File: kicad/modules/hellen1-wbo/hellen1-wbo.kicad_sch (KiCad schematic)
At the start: 65 parts, among them J600 Conn_02x03_Odd_Even, M600 Module-wbo-0.4, Q600 BTS3028, Q601 VNP28N04-E, U600 MCP6004, U601 AD8628, U602 STM32F042K6Tx, U603 REF3033, U604 XC6206P332MR, U605 TJA1051T/3/1J

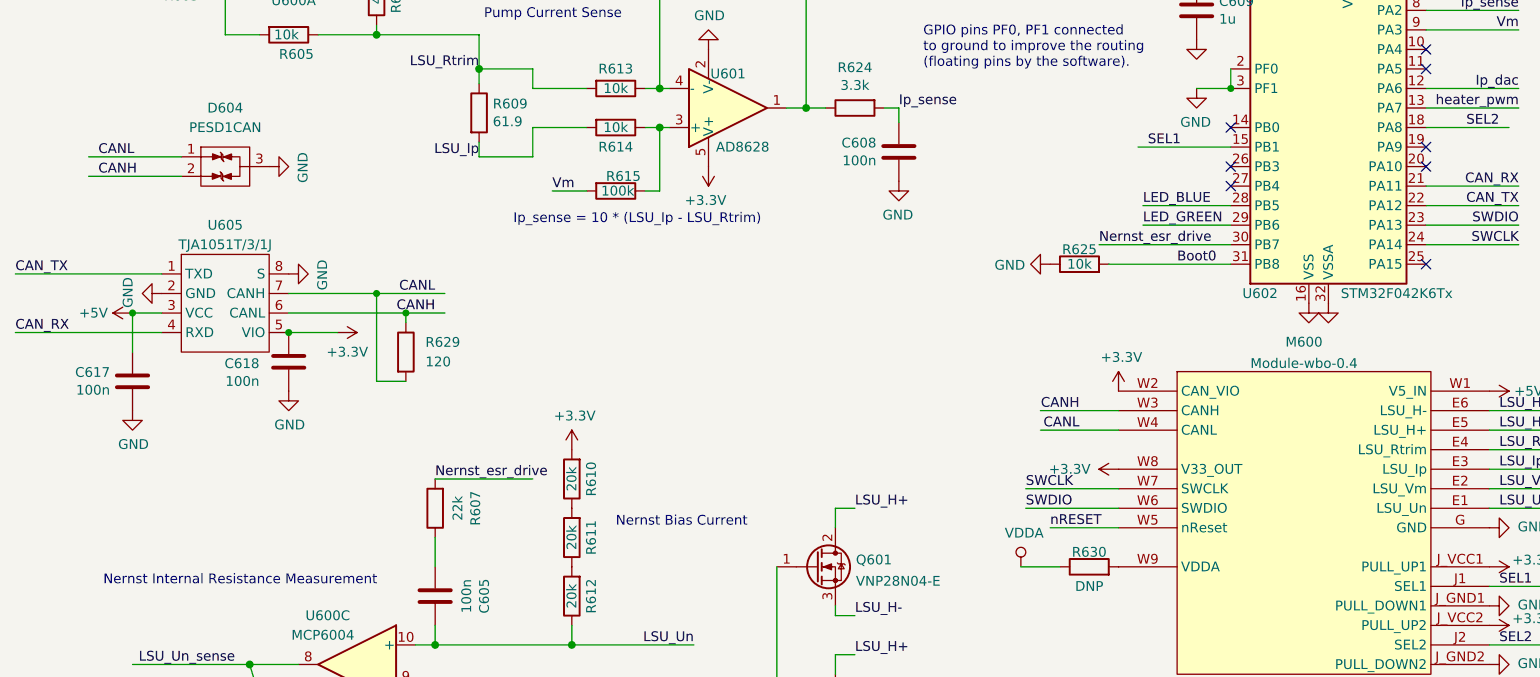
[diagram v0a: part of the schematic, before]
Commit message: rev.0.5
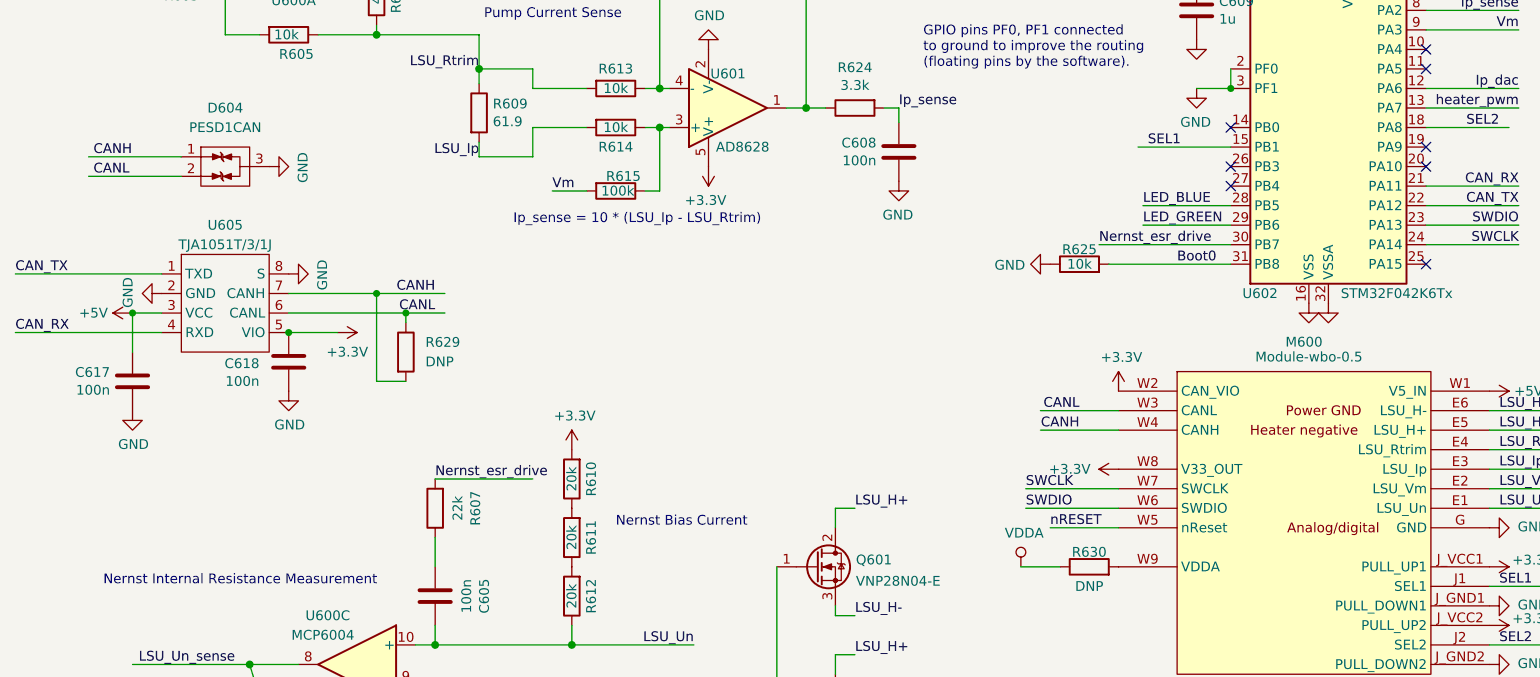
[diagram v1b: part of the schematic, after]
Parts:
- M600: value Module-wbo-0.4 -> Module-wbo-0.5; symbol hellen-one-wbo-0.4:Module-wbo-0.4 -> hellen-one-wbo-0.5:Module-wbo-0.5
- R629: value 120 -> DNP; LCSC C25079 -> (none)
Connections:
- net CANH: now also D604.1 (G), M600.W4 (CANH), R629.2, U605.7 (CANH); no longer D604.2 (D), M600.W3 (CANH), R629.1, U605.6 (CANL)
- net CANL: now also D604.2 (D), M600.W3 (CANL), R629.1, U605.6 (CANL); no longer D604.1 (G), M600.W4 (CANL), R629.2, U605.7 (CANH)
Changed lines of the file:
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@@
     (title "WBO")
     (date "2021-09-28")
-    (rev "0.3")
+    (rev "0.5")
     (company "rusefi.com")
   )
@@
     (effects (font (size 1.27 1.27)) (justify left bottom))
   )
-  (label "CANH" (at 72.39 114.3 180)
+  (label "CANH" (at 72.39 111.76 180)
     (effects (font (size 1.27 1.27)) (justify right bottom))
   )
@@
     (effects (font (size 1.27 1.27)) (justify right bottom))
   )
-  (label "CANH" (at 28.575 96.52 0)
+  (label "CANH" (at 27.94 93.98 0)
     (effects (font (size 1.27 1.27)) (justify left bottom))
   )
@@
     (effects (font (size 1.27 1.27)) (justify left bottom))
   )
-  (label "CANL" (at 28.575 93.98 0)
+  (label "CANL" (at 27.94 96.52 0)
     (effects (font (size 1.27 1.27)) (justify left bottom))
   )
@@
     (effects (font (size 1.27 1.27)) (justify right bottom))
   )
-  (label "CANH" (at 156.21 127 180)
+  (label "CANH" (at 156.21 129.54 180)
     (effects (font (size 1.27 1.27)) (justify right bottom))
   )
-  (label "CANL" (at 72.39 111.76 180)
+  (label "CANL" (at 72.39 114.3 180)
     (effects (font (size 1.27 1.27)) (justify right bottom))
   )
@@
     (effects (font (size 1.27 1.27)) (justify left bottom))
   )
-  (label "CANL" (at 156.21 129.54 180)
+  (label "CANL" (at 156.21 127 180)
     (effects (font (size 1.27 1.27)) (justify right bottom))
   )
@@
     (pin "1")
   )
-  (symbol (lib_id "hellen-one-wbo-0.4:Module-wbo-0.4") (at 168.91 121.92 0) (unit 1)
-    (in_bom yes) (on_board yes) (fields_autoplaced)
+  (symbol (lib_id "hellen-one-wbo-0.5:Module-wbo-0.5") (at 168.91 121.92 0) (unit 1)
+    (in_bom yes) (on_board yes)
     (property "Reference" "M600" (id 0) (at 185.42 118.0804 0))
-    (property "Value" "Module-wbo-0.4" (id 1) (at 185.42 120.8555 0))
+    (property "Value" "Module-wbo-0.5" (id 1) (at 186.055 120.015 0))
     (property "Footprint" "hellen-one-wbo-0.4:wbo" (id 2) (at 194.31 120.65 0)
       (effects (font (size 1.27 1.27)) hide)
@@
       (effects (font (size 1.27 1.27)) (justify left))
     )
-    (property "Value" "120" (id 1) (at 71.12 120.65 0)
+    (property "Value" "DNP" (id 1) (at 71.12 120.65 0)
       (effects (font (size 1.27 1.27)) (justify left))
     )
@@
       (effects (font (size 1.27 1.27)) hide)
     )
-    (property "LCSC" "C25079" (id 4) (at 68.58 119.38 0)
+    (property "LCSC" "" (id 4) (at 68.58 119.38 0)
       (effects (font (size 1.27 1.27)) hide)
     )
@@
     )
     (path "/b31bd6a2-d597-4ef3-ad7d-f0d5e79bcc1c"
-      (reference "M600") (unit 1) (value "Module-wbo-0.4") (footprint "hellen-one-wbo-0.4:wbo")
+      (reference "M600") (unit 1) (value "Module-wbo-0.5") (footprint "hellen-one-wbo-0.4:wbo")
     )
     (path "/00000000-0000-0000-0000-0000600e1a2d"
@@
     )
     (path "/b9ed5c9f-08c2-46c3-9f49-260a5ce30362"
-      (reference "R629") (unit 1) (value "120") (footprint "Resistor_SMD:R_0402_1005Metric")
+      (reference "R629") (unit 1) (value "DNP") (footprint "Resistor_SMD:R_0402_1005Metric")
     )
     (path "/8719995c-7a59-4520-a953-b0d876dea9a1"

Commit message: Revert "rev.0.5"
This reverts commit b22bcf23b6024c6822f90be4ccf93951eb7eb129.
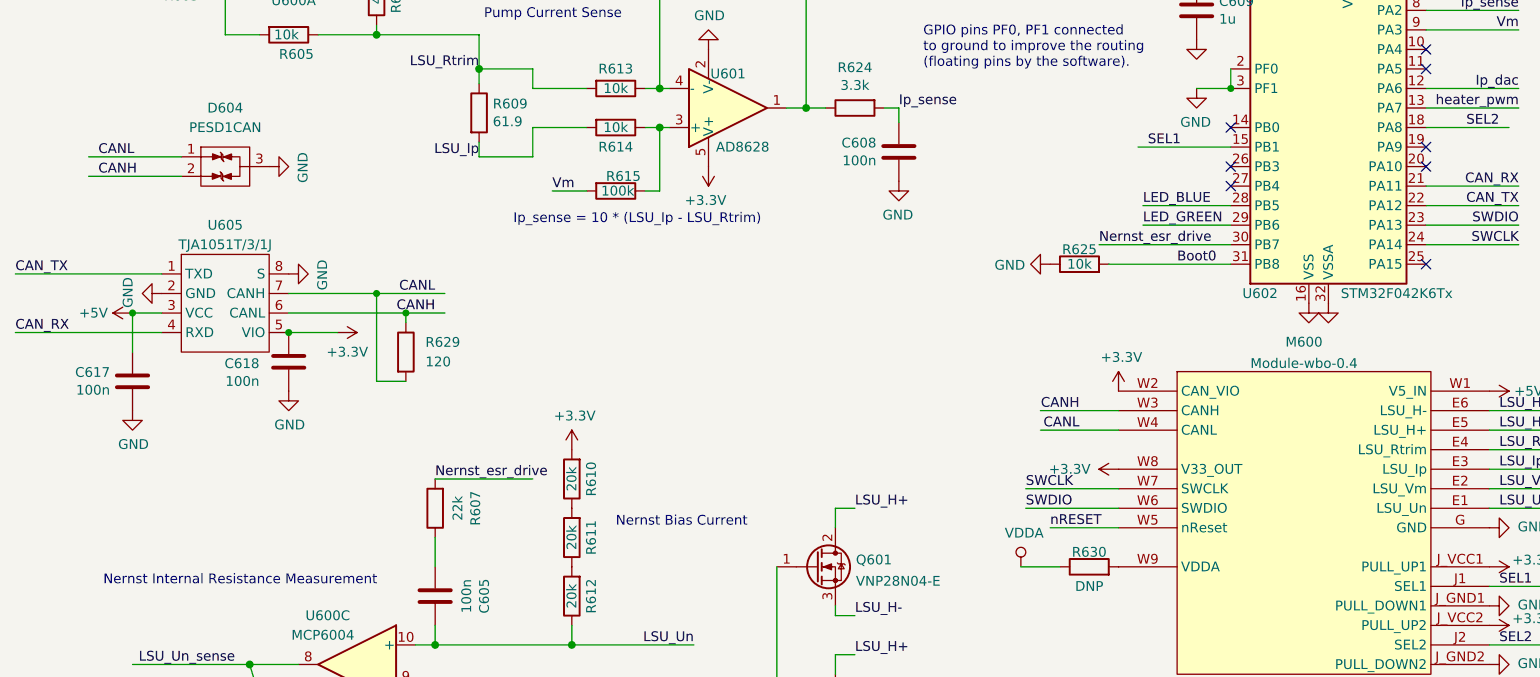
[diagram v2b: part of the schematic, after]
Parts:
- M600: value Module-wbo-0.5 -> Module-wbo-0.4; symbol hellen-one-wbo-0.5:Module-wbo-0.5 -> hellen-one-wbo-0.4:Module-wbo-0.4
- R629: value DNP -> 120; LCSC (none) -> C25079
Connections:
- net CANH: now also D604.2 (D), M600.W3 (CANH), R629.1, U605.6 (CANL); no longer D604.1 (G), M600.W4 (CANH), R629.2, U605.7 (CANH)
- net CANL: now also D604.1 (G), M600.W4 (CANL), R629.2, U605.7 (CANH); no longer D604.2 (D), M600.W3 (CANL), R629.1, U605.6 (CANL)
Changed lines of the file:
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@@
     (title "WBO")
     (date "2021-09-28")
-    (rev "0.5")
+    (rev "0.3")
     (company "rusefi.com")
   )
@@
     (effects (font (size 1.27 1.27)) (justify left bottom))
   )
-  (label "CANH" (at 72.39 111.76 180)
+  (label "CANH" (at 72.39 114.3 180)
     (effects (font (size 1.27 1.27)) (justify right bottom))
   )
@@
     (effects (font (size 1.27 1.27)) (justify right bottom))
   )
-  (label "CANH" (at 27.94 93.98 0)
+  (label "CANH" (at 28.575 96.52 0)
     (effects (font (size 1.27 1.27)) (justify left bottom))
   )
@@
     (effects (font (size 1.27 1.27)) (justify left bottom))
   )
-  (label "CANL" (at 27.94 96.52 0)
+  (label "CANL" (at 28.575 93.98 0)
     (effects (font (size 1.27 1.27)) (justify left bottom))
   )
@@
     (effects (font (size 1.27 1.27)) (justify right bottom))
   )
-  (label "CANH" (at 156.21 129.54 180)
+  (label "CANH" (at 156.21 127 180)
     (effects (font (size 1.27 1.27)) (justify right bottom))
   )
-  (label "CANL" (at 72.39 114.3 180)
+  (label "CANL" (at 72.39 111.76 180)
     (effects (font (size 1.27 1.27)) (justify right bottom))
   )
@@
     (effects (font (size 1.27 1.27)) (justify left bottom))
   )
-  (label "CANL" (at 156.21 127 180)
+  (label "CANL" (at 156.21 129.54 180)
     (effects (font (size 1.27 1.27)) (justify right bottom))
   )
@@
     (pin "1")
   )
-  (symbol (lib_id "hellen-one-wbo-0.5:Module-wbo-0.5") (at 168.91 121.92 0) (unit 1)
-    (in_bom yes) (on_board yes)
+  (symbol (lib_id "hellen-one-wbo-0.4:Module-wbo-0.4") (at 168.91 121.92 0) (unit 1)
+    (in_bom yes) (on_board yes) (fields_autoplaced)
     (property "Reference" "M600" (id 0) (at 185.42 118.0804 0))
-    (property "Value" "Module-wbo-0.5" (id 1) (at 186.055 120.015 0))
+    (property "Value" "Module-wbo-0.4" (id 1) (at 185.42 120.8555 0))
     (property "Footprint" "hellen-one-wbo-0.4:wbo" (id 2) (at 194.31 120.65 0)
       (effects (font (size 1.27 1.27)) hide)
@@
       (effects (font (size 1.27 1.27)) (justify left))
     )
-    (property "Value" "DNP" (id 1) (at 71.12 120.65 0)
+    (property "Value" "120" (id 1) (at 71.12 120.65 0)
       (effects (font (size 1.27 1.27)) (justify left))
     )
@@
       (effects (font (size 1.27 1.27)) hide)
     )
-    (property "LCSC" "" (id 4) (at 68.58 119.38 0)
+    (property "LCSC" "C25079" (id 4) (at 68.58 119.38 0)
       (effects (font (size 1.27 1.27)) hide)
     )
@@
     )
     (path "/b31bd6a2-d597-4ef3-ad7d-f0d5e79bcc1c"
-      (reference "M600") (unit 1) (value "Module-wbo-0.5") (footprint "hellen-one-wbo-0.4:wbo")
+      (reference "M600") (unit 1) (value "Module-wbo-0.4") (footprint "hellen-one-wbo-0.4:wbo")
     )
     (path "/00000000-0000-0000-0000-0000600e1a2d"
@@
     )
     (path "/b9ed5c9f-08c2-46c3-9f49-260a5ce30362"
-      (reference "R629") (unit 1) (value "DNP") (footprint "Resistor_SMD:R_0402_1005Metric")
+      (reference "R629") (unit 1) (value "120") (footprint "Resistor_SMD:R_0402_1005Metric")
     )
     (path "/8719995c-7a59-4520-a953-b0d876dea9a1"
